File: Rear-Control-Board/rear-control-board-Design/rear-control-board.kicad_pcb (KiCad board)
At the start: 2 copper layers, 57 parts, among them J1 Conn_01x23, J2 Conn_01x23, J3 Conn_01x08, J4 JST-B2B-VERT-2PIN, J5 JST-B2B-VERT-2PIN, J6 Conn_01x02, J7 Micro_SD_Card, K1 T9VV1K15-12S, K2 G5V-2, K3 G5V-2, Q1 B5584, Q2 PSMN5R2-60YL, Q3 PSMN5R2-60YL, Q4 PSMN5R2-60YL, U1 Dev_Board_C, U2 TS2940CP33 ROG, U4 MAX33054EASA+T

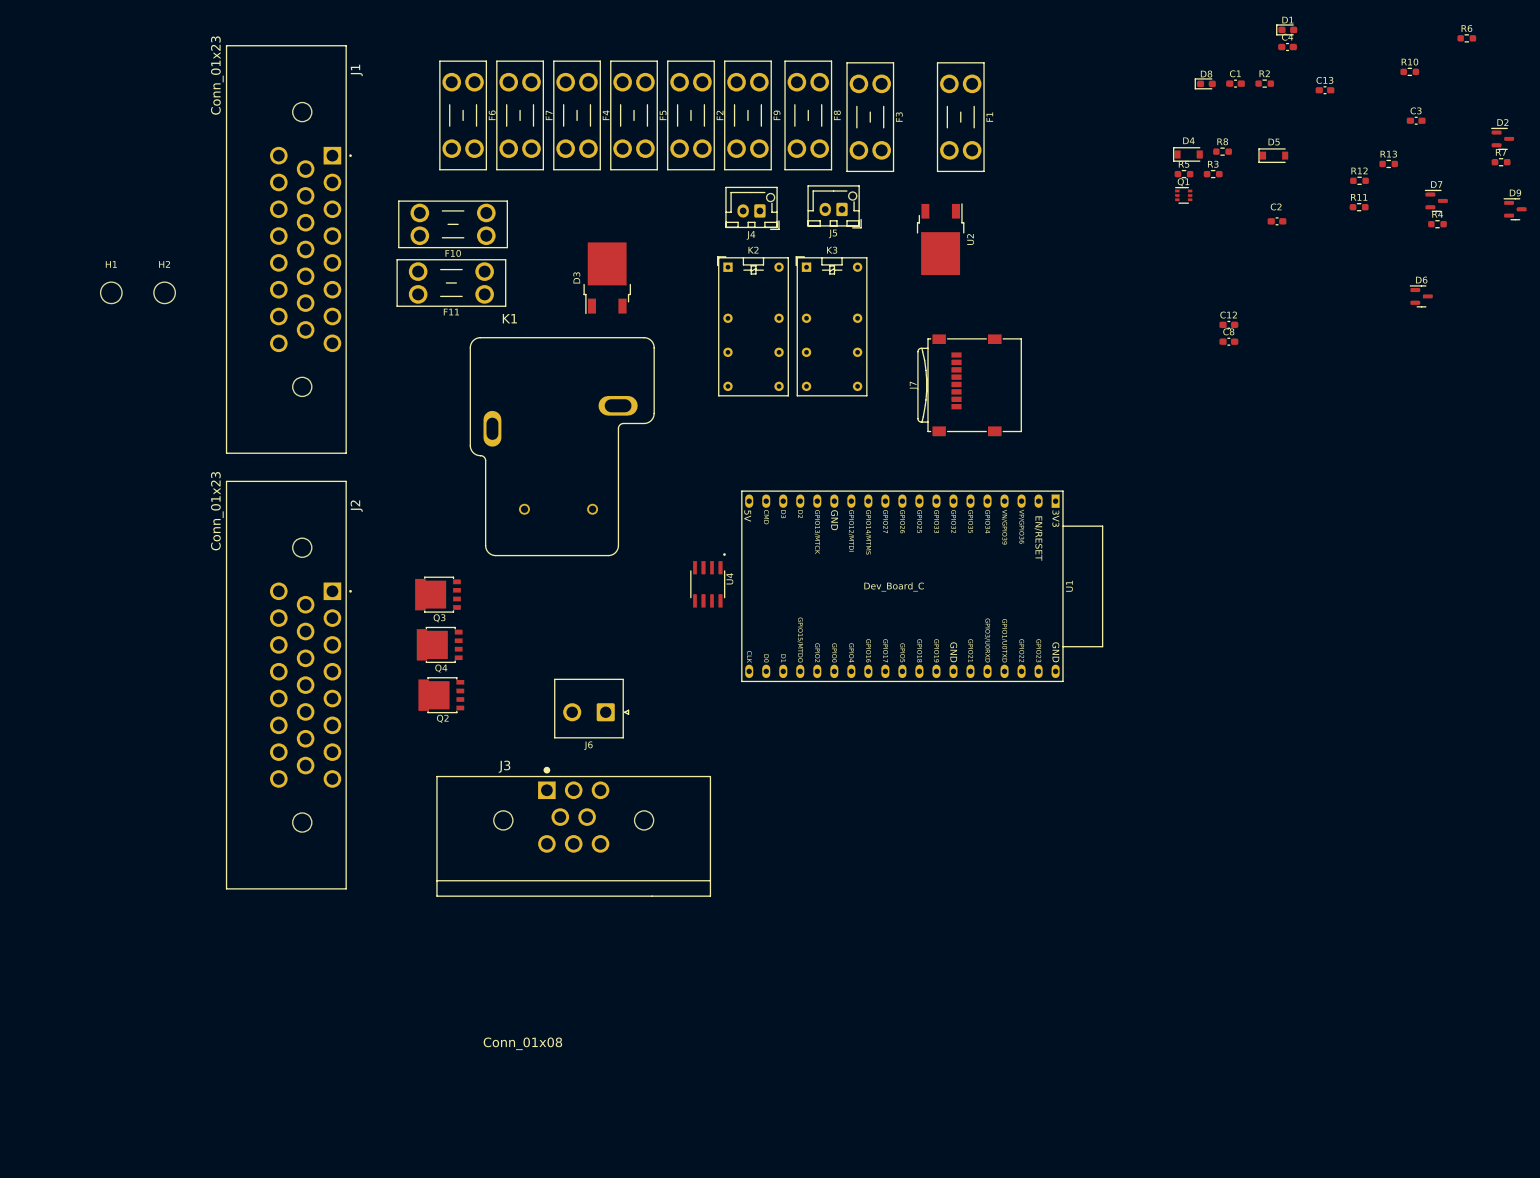
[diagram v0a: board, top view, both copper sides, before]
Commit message: commit
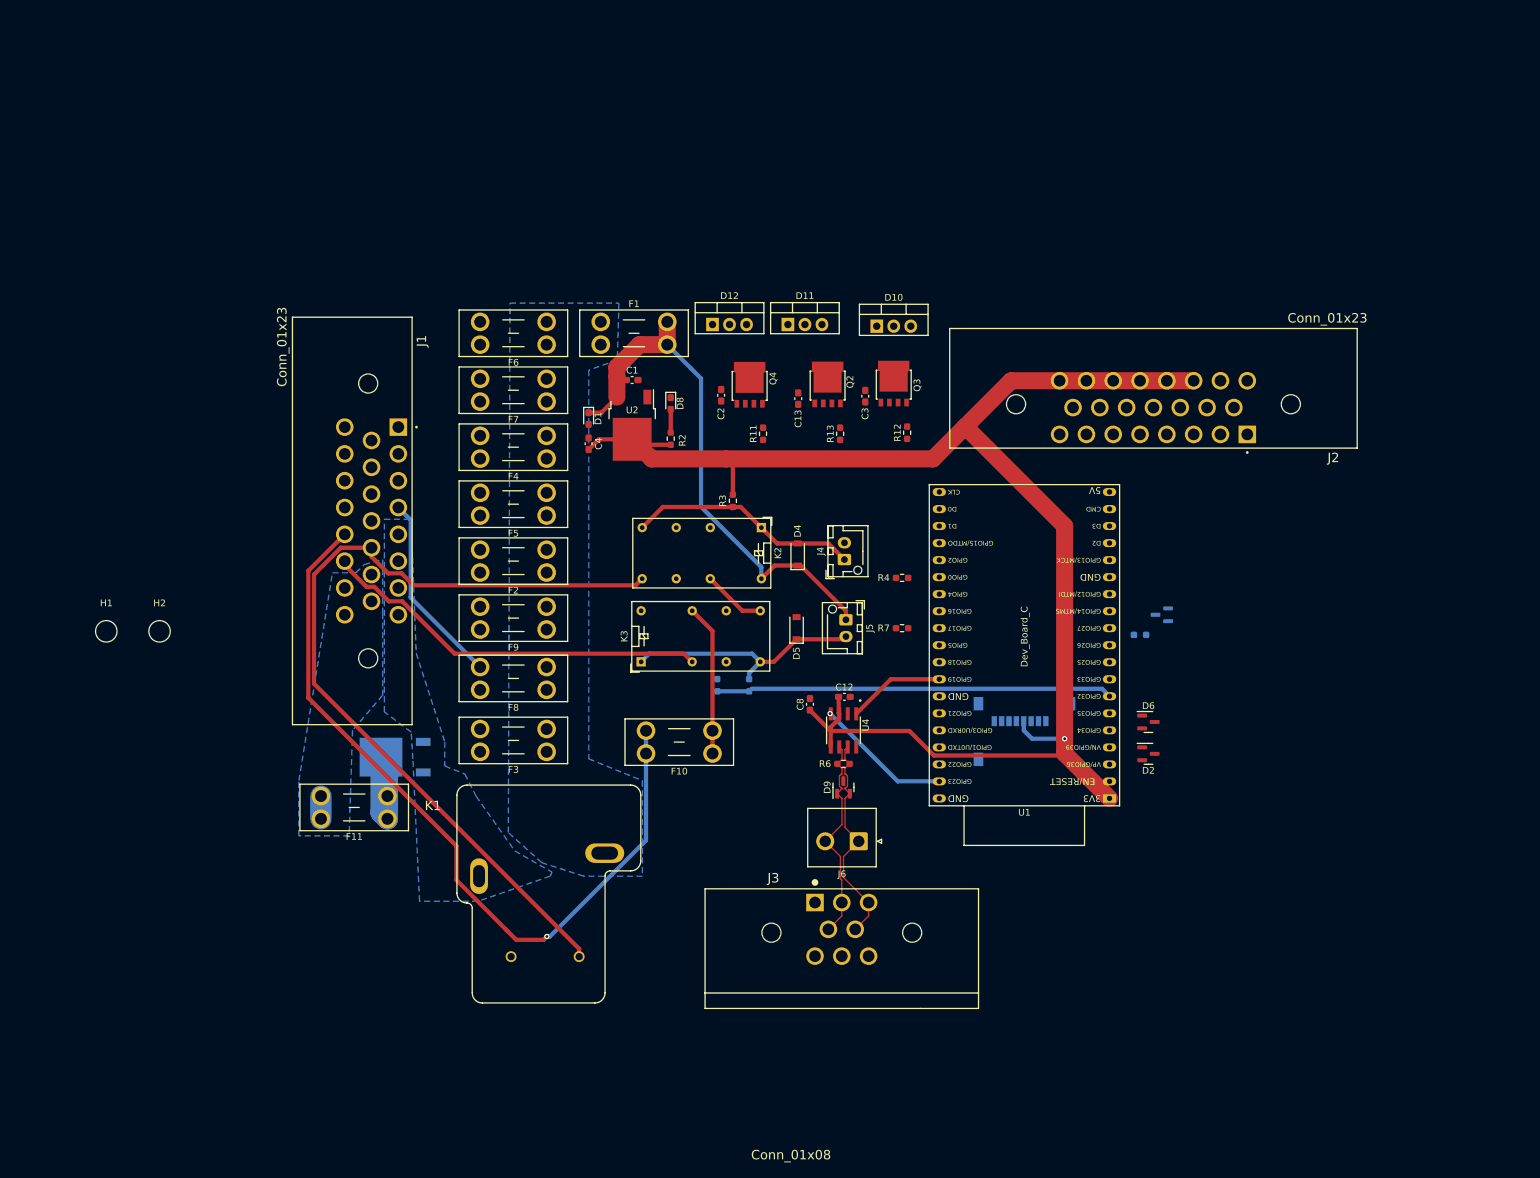
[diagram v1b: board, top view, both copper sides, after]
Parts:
- removed Q1: B5584, Package_TO_SOT_SMD:SOT-363_SC-70-6
- added D10: FERD20M60ST, Package_TO_SOT_THT:TO-220-3_Vertical, F.Cu at (155.2, 67.9)
- added D11: FERD20M60ST, Package_TO_SOT_THT:TO-220-3_Vertical, F.Cu at (142.0, 67.7)
- added D12: FERD20M60ST, Package_TO_SOT_THT:TO-220-3_Vertical, F.Cu at (130.7, 67.7)
- D3, D7, J7, R10, R5, R8: moved to B.Cu
- moved R6 142.7 mm to (150.2, 133.2), turned to 180 degrees
- moved J2 138.5 mm to (210.5, 84.1), turned to 180 degrees
- moved D9 132.2 mm to (150.2, 136.8), turned to 90 degrees
- moved C4 119.9 mm to (112.2, 85.5), turned to 90 degrees
- moved D1 119.4 mm to (112.2, 81.7), turned to -90 degrees
- moved R7 113.2 mm to (159.0, 113.0), turned to 180 degrees
- moved F3 111.5 mm to (106.0, 131.4), turned to 180 degrees
- moved R8 109.6 mm to (131.4, 121.5), turned to 90 degrees
- moved D2 105.9 mm to (195.8, 131.8)
- moved R2 103.3 mm to (124.5, 84.7), turned to 90 degrees
- moved C1 100.3 mm to (118.7, 76.0)
- moved D5 100.2 mm to (143.2, 113.0), turned to 90 degrees
- moved R5 100.1 mm to (136.2, 121.5), turned to -90 degrees
- moved F8 99.4 mm to (106.0, 122.2), turned to 180 degrees
- moved R4 95.7 mm to (159.0, 105.5), turned to 180 degrees
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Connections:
- F10 pad 2: /FuseBank/TSV -> /TSV
- F5 pad 2: /FuseBank/BMS_12V -> BMS_12V
- J1 pad 12: /BATT_12V -> /FAULT_BMS
- J1 pad 13: /BATT_12V -> /BRB_RTN
- J1 pad 20: /BRB_RTN -> /TSV
- J1 pad 22: /FAULT_BMS -> /DCDC_IN
- J1 pad 23: /FuseBank/TSV -> /DCDC_IN
- J1 pad 7: /DCDC_IN -> /BATT_12V
- J1 pad 8: /DCDC_IN -> /BATT_12V
- J2 pad 12: unconnected-(J2-Pad12) -> BMS_12V
- J2 pad 15: /WATER_IN- -> /WATER_OUT-
- J2 pad 8: /WATER_OUT- -> /WATER_IN-
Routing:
- net VDD: track 0.00 -> 230.2 mm, vias 0 -> 1
- net /BRB_RTN: track 0.00 -> 127.5 mm
- net /TSV: track 0.00 -> 117.5 mm, vias 0 -> 1
- net INT_12V: track 0.00 -> 81.9 mm
- net /Controller/FAULT_IMD: track 0.00 -> 59.2 mm
- net /FAULT_IMD: track 0.00 -> 58.4 mm
- net /FAULT_LATCHER/IMD_SWITCH: track 0.00 -> 36.4 mm
- net /FAULT_LATCHER/BMS_IND: track 0.00 -> 34.7 mm
- net /CAN_P: track 0.00 -> 33.2 mm
- net /CAN_N: track 0.00 -> 31.9 mm
- net /BRAKE_12V: track 0.00 -> 28.9 mm
- net /SSOK: track 0.00 -> 22.6 mm
- net /Controller/CAN_MOSI: track 0.00 -> 20.6 mm, vias 0 -> 1
- net /charge-controller/dcdc_fuse: track 0.00 -> 19.2 mm
- net /Controller/CAN_MISO: track 0.00 -> 14.5 mm
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- added copper zone on B.Cu, net +12V
- added copper zone on B.Cu, net /BATT_12V
- added copper zone on B.Cu, net /DCDC_IN

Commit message: update
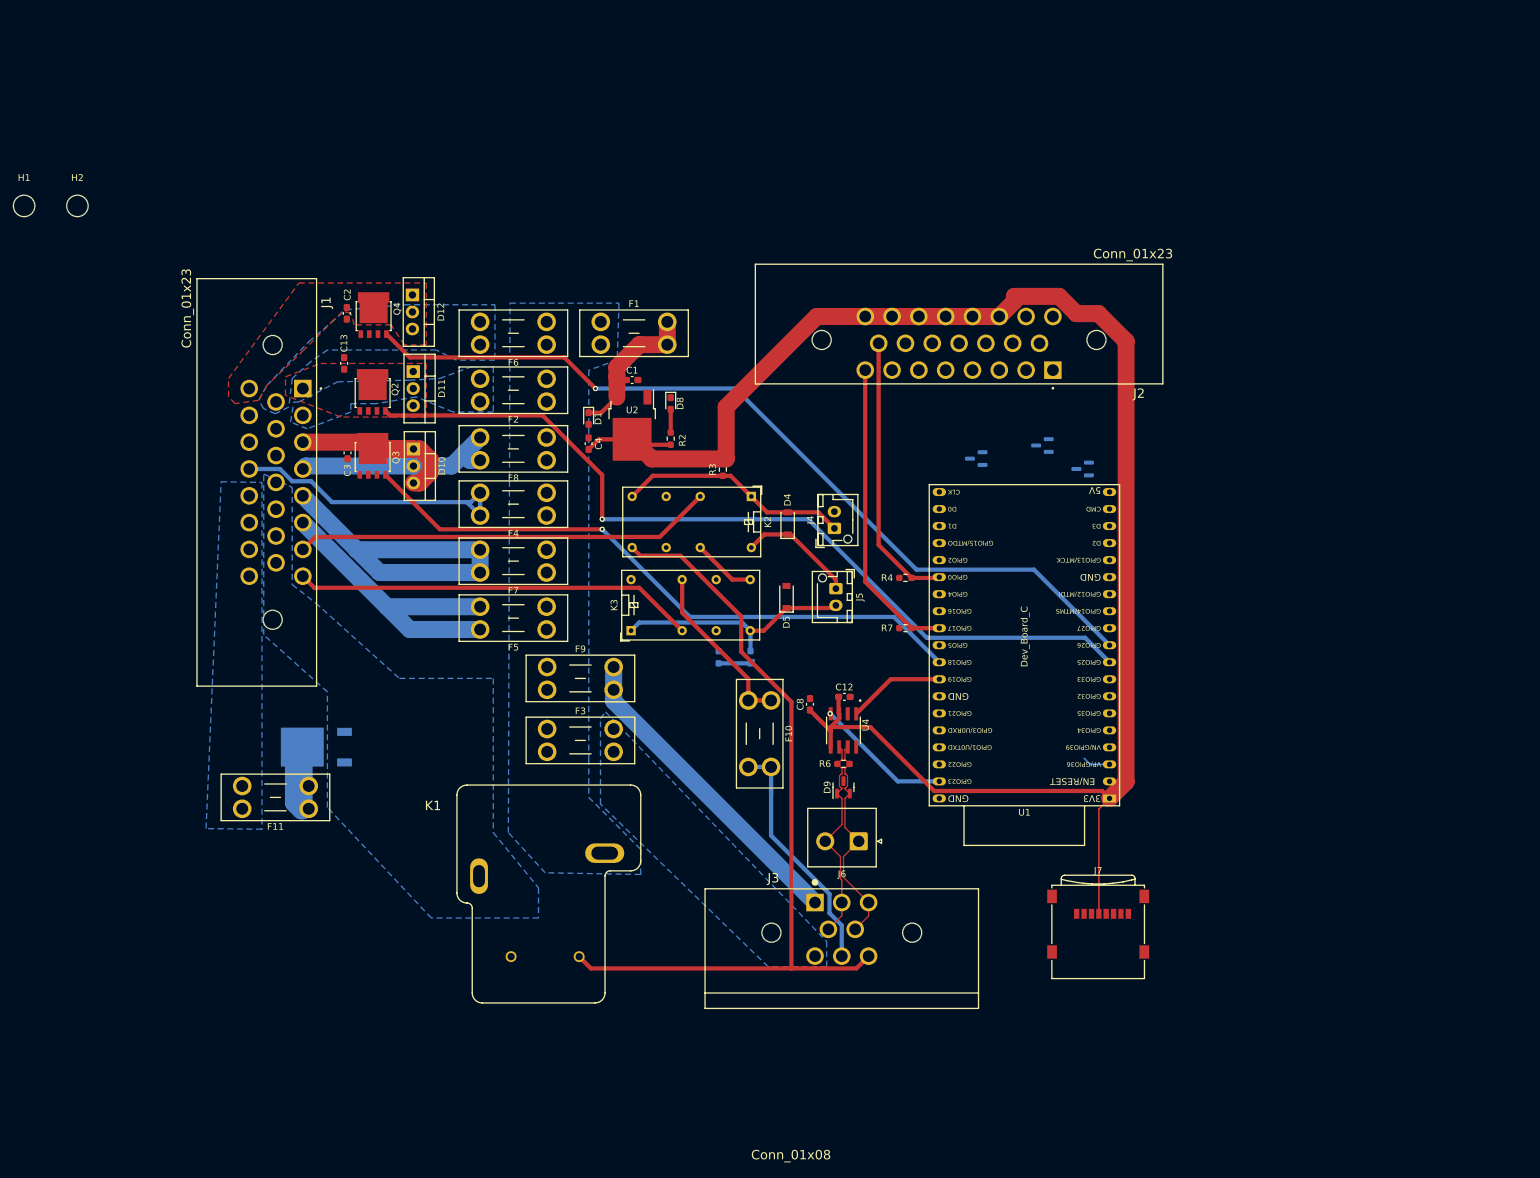
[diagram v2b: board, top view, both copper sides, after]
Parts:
- removed R10: 470, Resistor_SMD:R_0603_1608Metric_Pad0.98x0.95mm_HandSolder
- removed R11, R12, R13: 1.5K, Resistor_SMD:R_0603_1608Metric_Pad0.98x0.95mm_HandSolder
- D2, D6: moved to B.Cu
- J7: moved to F.Cu
- moved Q3 78.5 mm to (80.0, 87.3)
- moved C3 77.7 mm to (76.2, 86.8)
- moved D10 71.5 mm to (86.1, 86.3), turned to -90 degrees
- moved C13 68.0 mm to (75.8, 73.5), turned to 90 degrees
- moved Q2 67.9 mm to (80.0, 77.8)
- moved H1 64.6 mm to (28.0, 50.0)
- moved H2 64.6 mm to (36.0, 50.0)
- moved C2 57.2 mm to (76.2, 66.0)
- moved Q4 57.1 mm to (80.2, 66.3)
- moved D11 56.3 mm to (86.1, 74.7), turned to -90 degrees
- moved D2 51.0 mm to (170.1, 87.7), turned to 180 degrees
- moved D12 45.0 mm to (85.9, 63.3), turned to -90 degrees
- moved D6 44.2 mm to (179.9, 85.8), turned to 180 degrees
- moved F8 34.2 mm to (106.0, 88.0)
- moved J7 30.8 mm to (188.2, 157.2), turned to 0 degrees
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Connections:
- net /FAULT_LATCHER/BMS_IND renamed /FAULT_LATCHER/BMS_SWITCH
- F3 pad 2: /FuseBank/RINE_12V -> /RINE_12
- F4 pad 2: /FuseBank/FRONT_12V -> /FRONT_12
- F7 pad 2: /FuseBank/HVB_12 -> /HVB_12
- F9 pad 2: /FuseBank/BRB_LOOP -> /BRB_LOOP
- J1 pad 1: /FuseBank/HVB_12 -> /FAN_RTRN_12V
- J1 pad 12: /FAULT_BMS -> /BATT_12V
- J1 pad 13: /BRB_RTN -> /BATT_12V
- J1 pad 14: /DCDC_IN -> /BATT_12V
- J1 pad 15: /DCDC_IN -> /BATT_12V
- J1 pad 16: /FuseBank/FRONT_12V -> /PUMP_RTRN_12V
- J1 pad 17: /FuseBank/BRB_LOOP -> GND
- J1 pad 19: GND -> /FRONT_12
- J1 pad 2: /PUMP_12V -> /FAN_12V
- J1 pad 20: /TSV -> /DCDC_IN
- J1 pad 21: /FAULT_IMD -> /DCDC_IN
- J1 pad 3: /FAN_12V -> /BRAKE_RTRN_12V
- J1 pad 5: /BATT_12V -> /HVB_12
- J1 pad 6: /BATT_12V -> BMS_12V
- J1 pad 7: /BATT_12V -> /FAULT_BMS
- J1 pad 8: /BATT_12V -> /FAULT_IMD
- J1 pad 9: /FuseBank/RINE_12V -> /PUMP_12V
- J2 pad 12: BMS_12V -> unconnected-(J2-Pad12)
- J2 pad 3: /BRAKE_RTRN_12V -> unconnected-(J2-Pad3)
- J2 pad 4: /FAN_RTRN_12V -> unconnected-(J2-Pad4)
- J2 pad 5: /PUMP_RTRN_12V -> unconnected-(J2-Pad5)
- J3 pad 1: unconnected-(J3-Pad1) -> /BRB_LOOP
- J3 pad 6: unconnected-(J3-Pad6) -> /RINE_12
- J3 pad 7: unconnected-(J3-Pad7) -> /TSV
- J3 pad 8: GND -> /BRB_RTN
- Q2 pad 4: Net-(Q2-Pad4) -> /Controller/BRAKE_CTRL
- Q3 pad 4: Net-(Q3-Pad4) -> /Controller/PUMP_CTRL
- Q4 pad 4: Net-(Q4-Pad4) -> /Controller/FAN_CTRL
- U1 pad 10: /Controller/BRAKE_CTRL -> /Controller/FAN_CTRL
- U1 pad 9: /Controller/FAN_CTRL -> /Controller/BRAKE_CTRL
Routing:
- net /Controller/BRAKE_CTRL: track 0.00 -> 127.4 mm, vias 0 -> 1
- net /Controller/FAN_CTRL: track 0.00 -> 127.1 mm, vias 0 -> 1
- net /Controller/PUMP_CTRL: track 0.00 -> 94.2 mm, vias 0 -> 1
- net /TSV: track 117.5 -> 36.7 mm, vias 1 -> 0
- net /FAULT_BMS: track 0.00 -> 62.6 mm
- net /Controller/FAULT_IMD: track 59.2 -> 5.29 mm
- net /HVB_12: track 0.00 -> 53.0 mm
- net /BRB_LOOP: track 0.00 -> 47.6 mm
- net BMS_12V: track 0.00 -> 47.0 mm
- net /WATER_IN-: track 0.00 -> 45.5 mm
- net /FRONT_12: track 0.00 -> 43.3 mm
- net /WATER_OUT-: track 0.00 -> 41.2 mm
- net INT_12V: track 81.9 -> 41.1 mm
- net /BRAKE_RTRN_12V: track 0.00 -> 30.2 mm
- net VDD: track 230.2 -> 251.5 mm, vias 1 -> 0
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- added copper zone on B.Cu, net /FAN_12V
- added copper zone on F.Cu, net /FAN_RTRN_12V
- added copper zone on B.Cu, net /PUMP_12V
- added copper zone on F.Cu, net /PUMP_RTRN_12V
- added copper zone on B.Cu, net /RINE_12
